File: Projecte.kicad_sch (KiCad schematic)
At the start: 1 part, among them U1 PIC18F448-IP

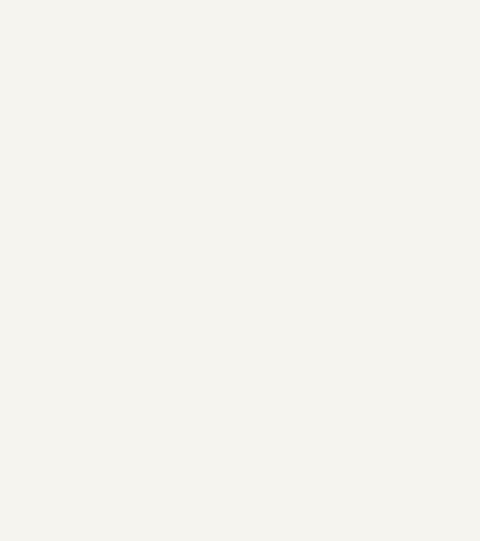
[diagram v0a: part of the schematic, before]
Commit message: Update Projecte.kicad_sch
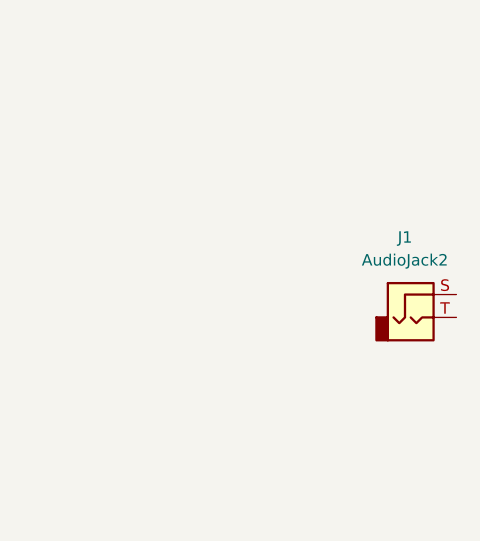
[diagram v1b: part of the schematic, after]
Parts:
- added J1: AudioJack2, symbol Connector_Audio:AudioJack2
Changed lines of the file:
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@@
 	(paper "A4")
+	(symbol
+		(lib_id "Connector_Audio:AudioJack2")
+		(at 238.76 95.25 0)
+		(unit 1)
+		(exclude_from_sim no)
+		(in_bom yes)
+		(on_board yes)
+		(dnp no)
+		(fields_autoplaced yes)
+		(property "Reference" "J1"
+			(at 238.125 86.36 0)
+			(effects
+				(font
+					(size 1.27 1.27)
+				)
+			)
+		)
+		(property "Value" "AudioJack2"
+			(at 238.125 88.9 0)
+			(effects
+				(font
+					(size 1.27 1.27)
+				)
+			)
+		)
+		(property "Footprint" ""
+			(at 238.76 95.25 0)
+			(effects
+				(font
+					(size 1.27 1.27)
+				)
+				(hide yes)
+			)
+		)
+		(property "Datasheet" "~"
+			(at 238.76 95.25 0)
+			(effects
+				(font
+					(size 1.27 1.27)
+				)
+				(hide yes)
+			)
+		)
+		(property "Description" "Audio Jack, 2 Poles (Mono / TS)"
+			(at 238.76 95.25 0)
+			(effects
+				(font
+					(size 1.27 1.27)
+				)
+				(hide yes)
+			)
+		)
+		(pin "S"
+		)
+		(pin "T"
+		)
+		(instances
+			(project ""
+				(path "/3a490218-d26e-483b-a44b-688997a15829"
+					(reference "J1")
+					(unit 1)
+				)
+			)
+		)
+	)
 	(symbol
 		(lib_id "MCU_Microchip_PIC18:PIC18F448-IP")
